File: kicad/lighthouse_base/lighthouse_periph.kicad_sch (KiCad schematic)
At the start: 7 parts, among them J3 Conn_01x12, J4 Conn_01x12, J5 Conn_01x06, J6 Conn_01x02

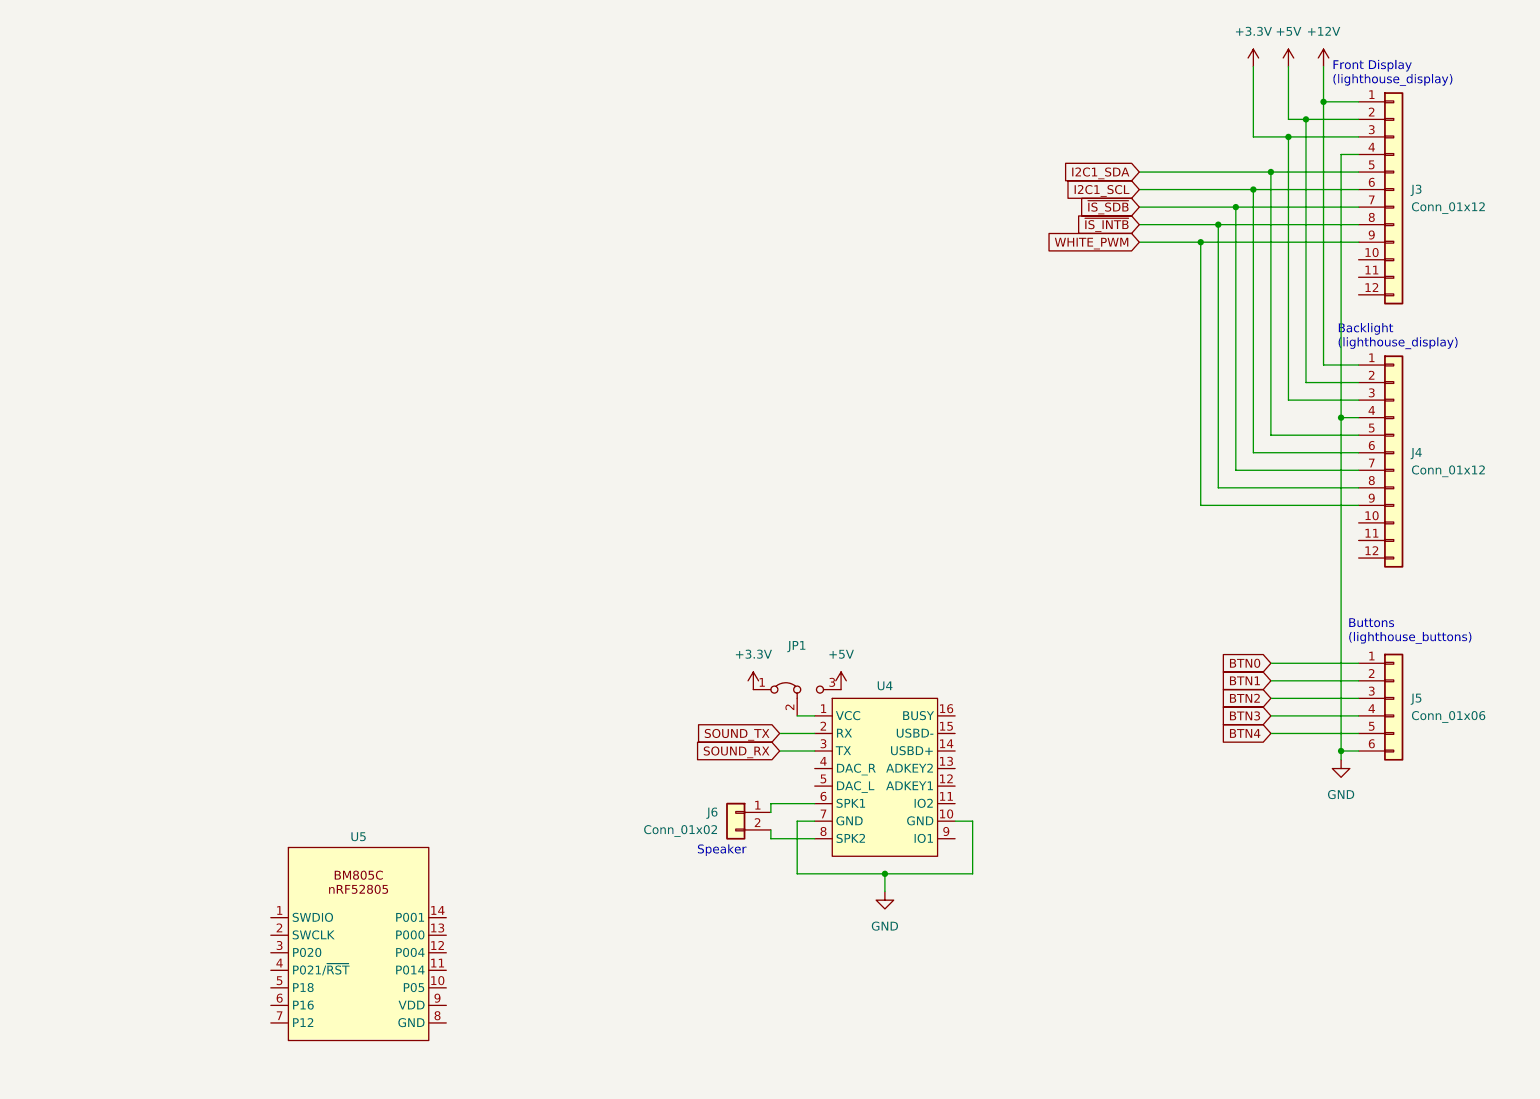
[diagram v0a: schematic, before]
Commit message: schema v1 done
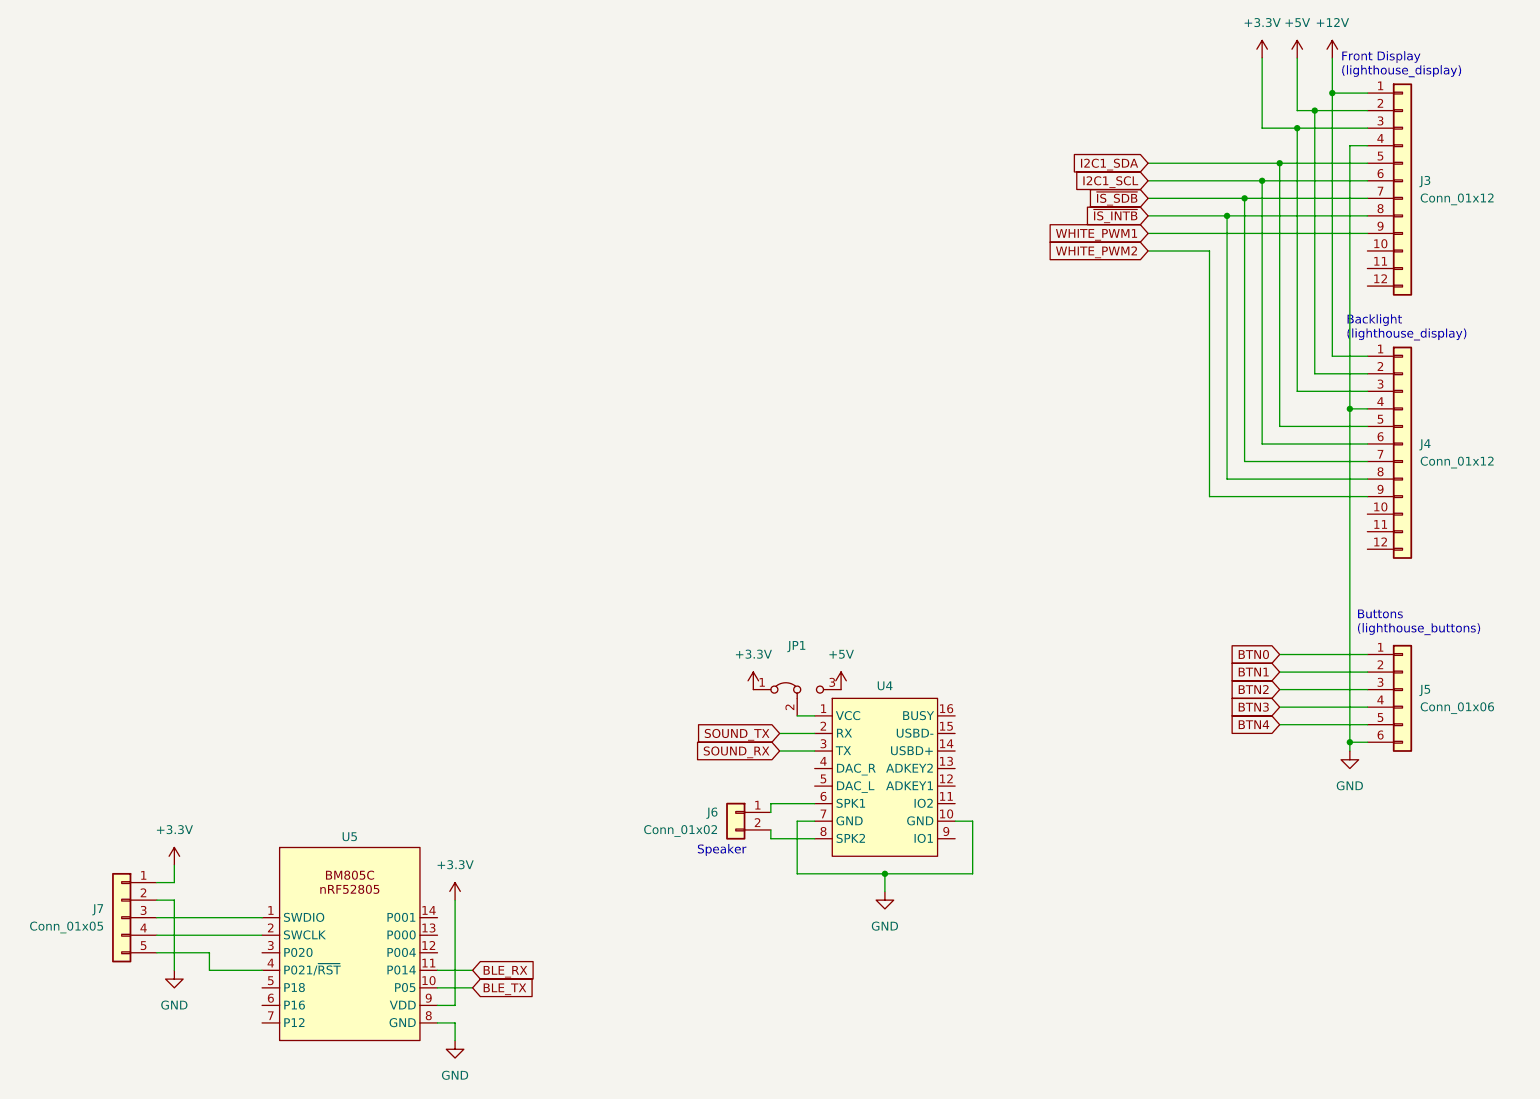
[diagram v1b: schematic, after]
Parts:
- added J7: Conn_01x05, symbol Connector_Generic:Conn_01x05
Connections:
- net +3.3V: now also U5.9 (VDD), J7.1 (Pin_1)
- net GND: now also U5.8 (GND), J7.2 (Pin_2)
- net at U5.1 (SWDIO): now also J7.3 (Pin_3)
- net BLE_TX: now reaches U5.10 (P05)
- net BLE_RX: now reaches U5.11 (P014)
- net at U5.2 (SWCLK): now also J7.4 (Pin_4)
- net at U5.4 (P021/~{RST}): now also J7.5 (Pin_5)
- net WHITE_PWM renamed WHITE_PWM1
- net WHITE_PWM1: no longer J4.9 (Pin_9)
- new net WHITE_PWM2: J4.9 (Pin_9)
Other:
- moved on the sheet: J3, J4, J5, U5
